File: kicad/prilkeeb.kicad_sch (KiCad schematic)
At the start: 71 parts, among them U2 Nice_Nano_V2

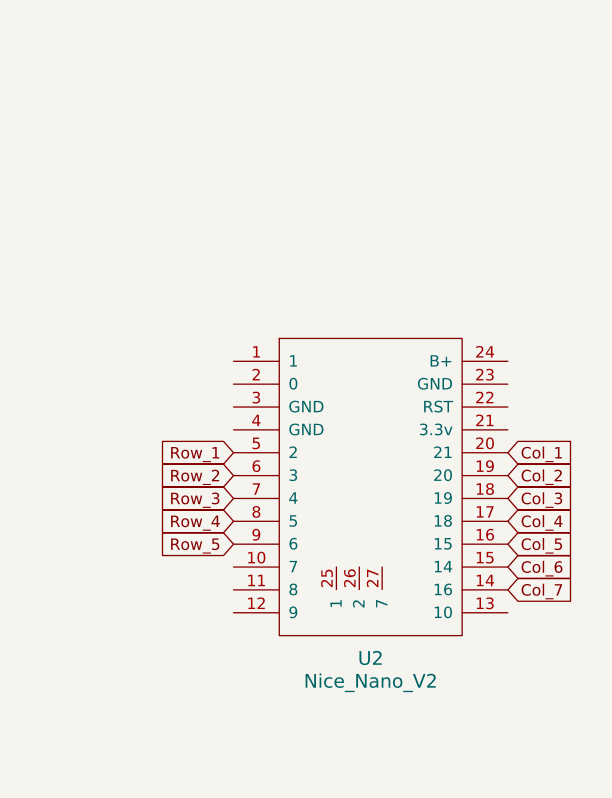
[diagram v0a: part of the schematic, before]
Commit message: Update design
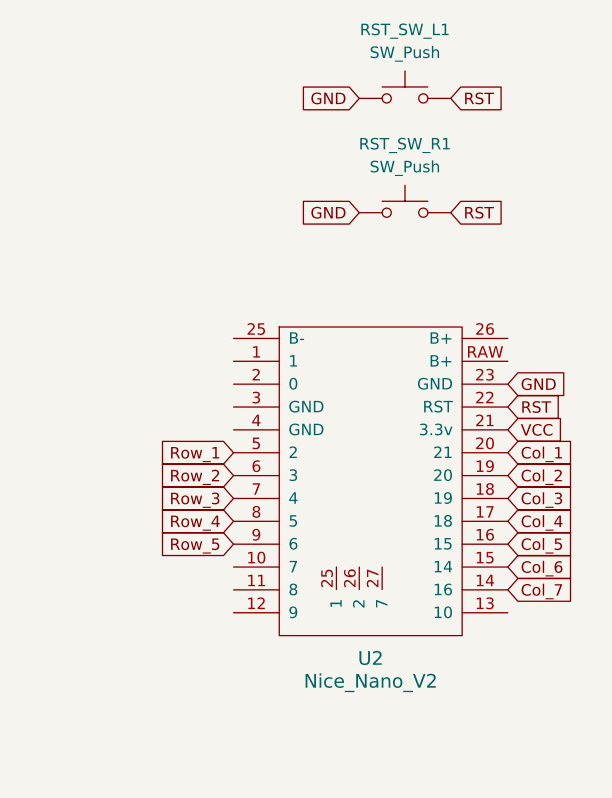
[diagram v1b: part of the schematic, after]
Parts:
- added RST_SW_L1, RST_SW_R1: SW_Push, Button_Switch_SMD:SW_SPST_SKQG_WithStem, symbol Switch:SW_Push
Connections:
- net VCC: now reaches U2.21 (3.3v)
- net RST: now reaches U2.22 (RST)
- net RST: now also RST_SW_L1.2, RST_SW_R1.2
- net GND: now reaches U2.23 (GND)
- net GND: now also RST_SW_L1.1, RST_SW_R1.1
